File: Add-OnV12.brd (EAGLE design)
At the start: 28.1 x 17.6 mm, 10 parts

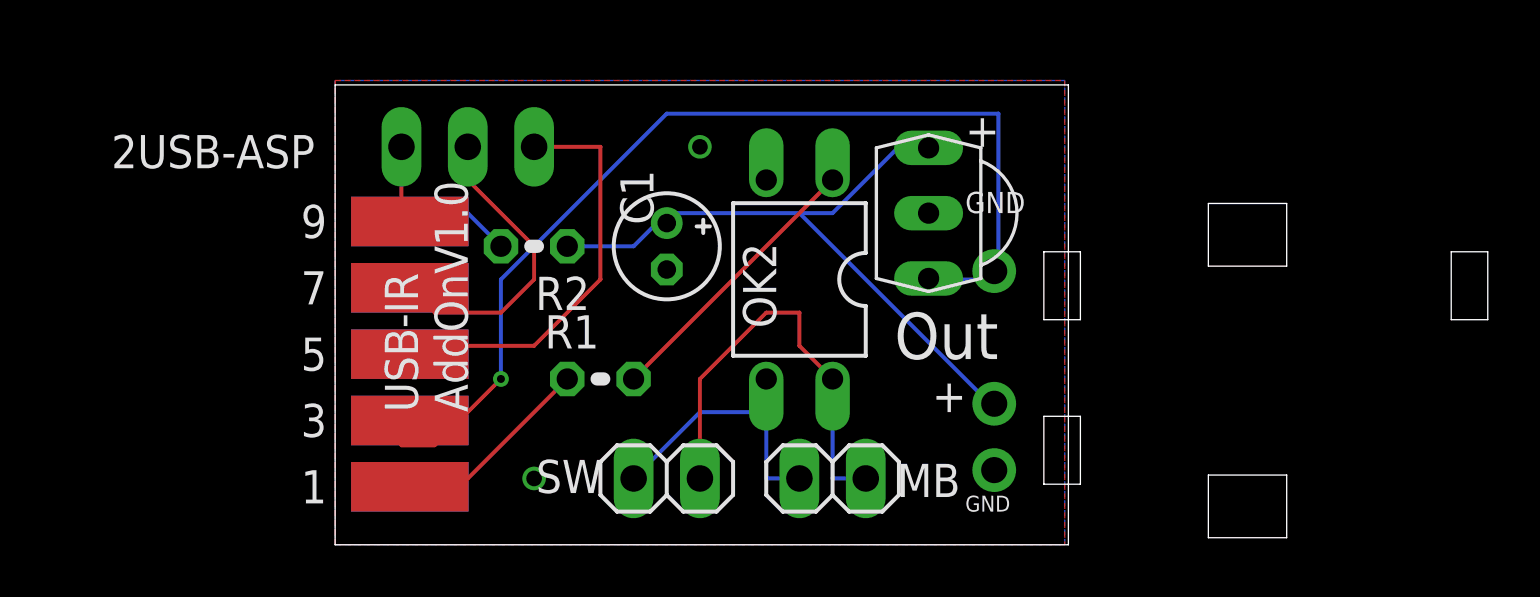
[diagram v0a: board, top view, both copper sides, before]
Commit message: Update
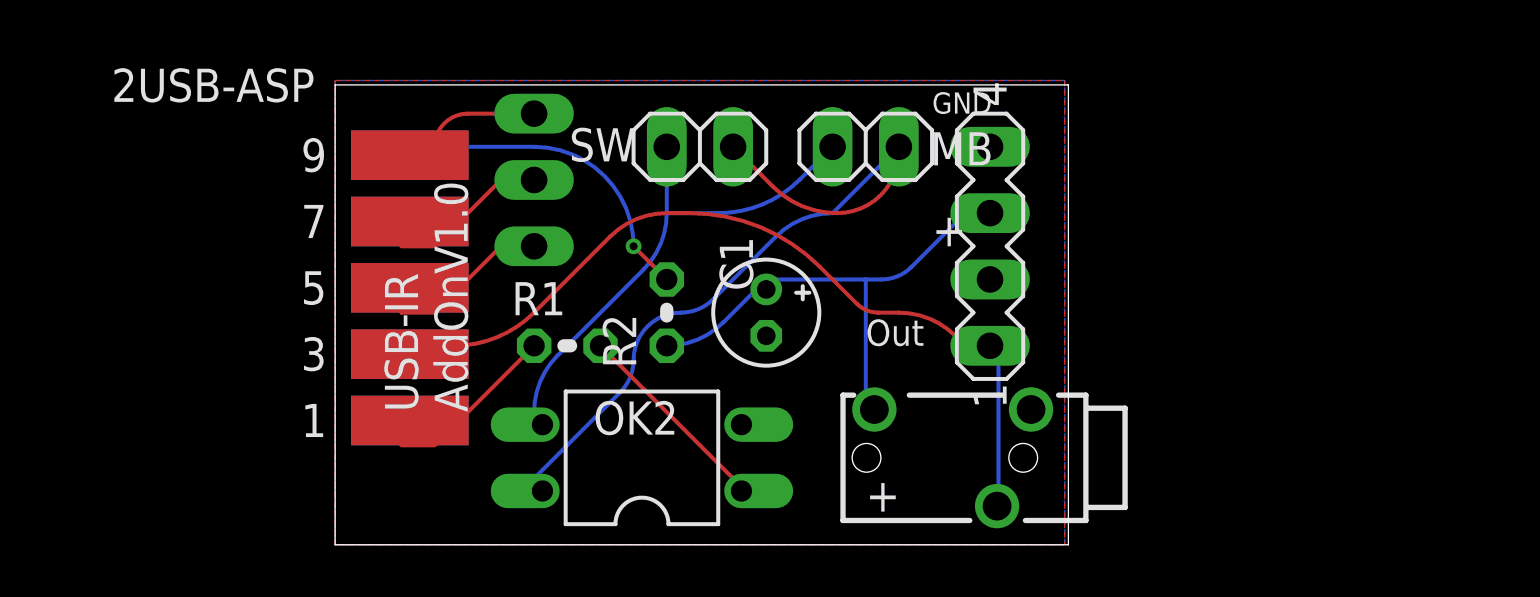
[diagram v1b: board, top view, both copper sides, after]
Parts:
- removed IR1: TSOP1738TB1, telefunken:TSOP17_TB1
- removed U$1: TSOP1838, tsop-1:TSOP18XX
- added SV1: (no value), con-lstb:MA04-1
- added X1: 1501_03, con-lumberg:1501_03
- moved MB 12.8 mm to (20.3, 15.2)
- moved SW 12.8 mm to (14.0, 15.2)
- moved OK2 9.11 mm to (11.8, 3.33), turned to 90 degrees
- moved R2 5.68 mm to (12.7, 8.89), turned to 90 degrees
- moved C1 4.58 mm to (16.5, 8.89)
- moved FREI 2.84 mm to (7.62, 14.0), turned to 270 degrees
- moved 2USB-ASP 2.54 mm to (2.86, 9.84)
- moved R1 1.80 mm to (8.89, 7.62)
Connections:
- net GND: now also SV1.4, X1.1; no longer IR1.GND, U$1.GND
- net N$1: now also SV1.3, X1.3; no longer IR1.VS, U$1.VCC
- net SCK: now also SV1.1, X1.2; no longer IR1.VO, U$1.OUT
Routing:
- net N$3: track 16.8 -> 28.2 mm
- net SCK: track 41.5 -> 32.2 mm, vias 1 -> 0
- net N$4: track 11.2 -> 19.6 mm
- net RST: track 16.0 -> 7.85 mm
- net VCC: track 4.07 -> 12.0 mm, vias 0 -> 1
- net N$1: track 26.9 -> 20.0 mm
- net NC: track 12.7 -> 7.85 mm
- net N$2: track 10.8 -> 7.76 mm
- net MOSI: track 2.99 -> 5.34 mm
- net MISO: track 7.66 -> 8.38 mm
